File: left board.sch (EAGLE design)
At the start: 35 parts, among them IC1 LM555D, IC2 LM555D, IC3 LM50, IC4 LM50

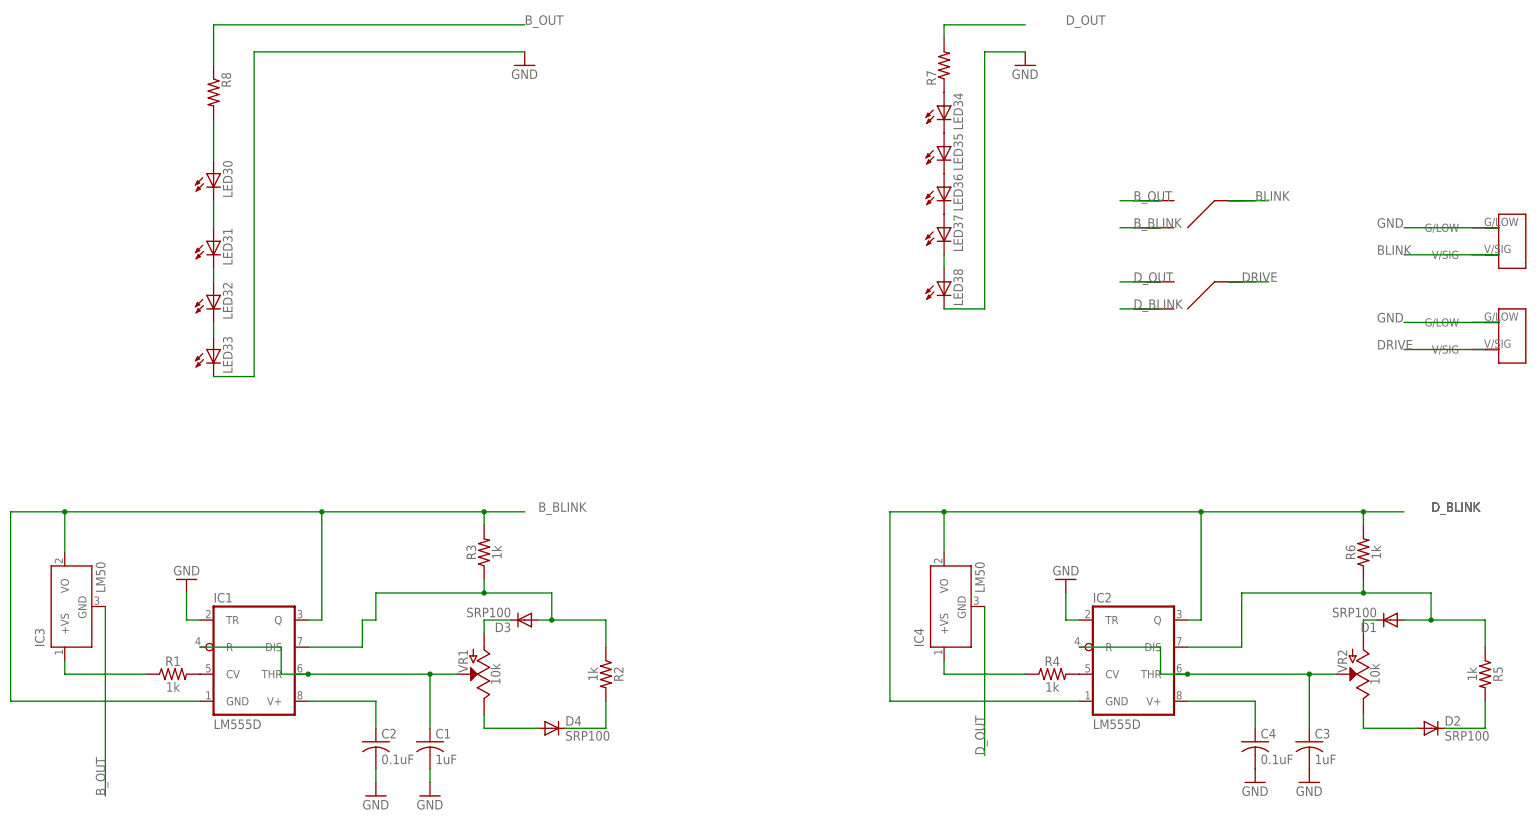
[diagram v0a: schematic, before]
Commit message: Gerbers generated
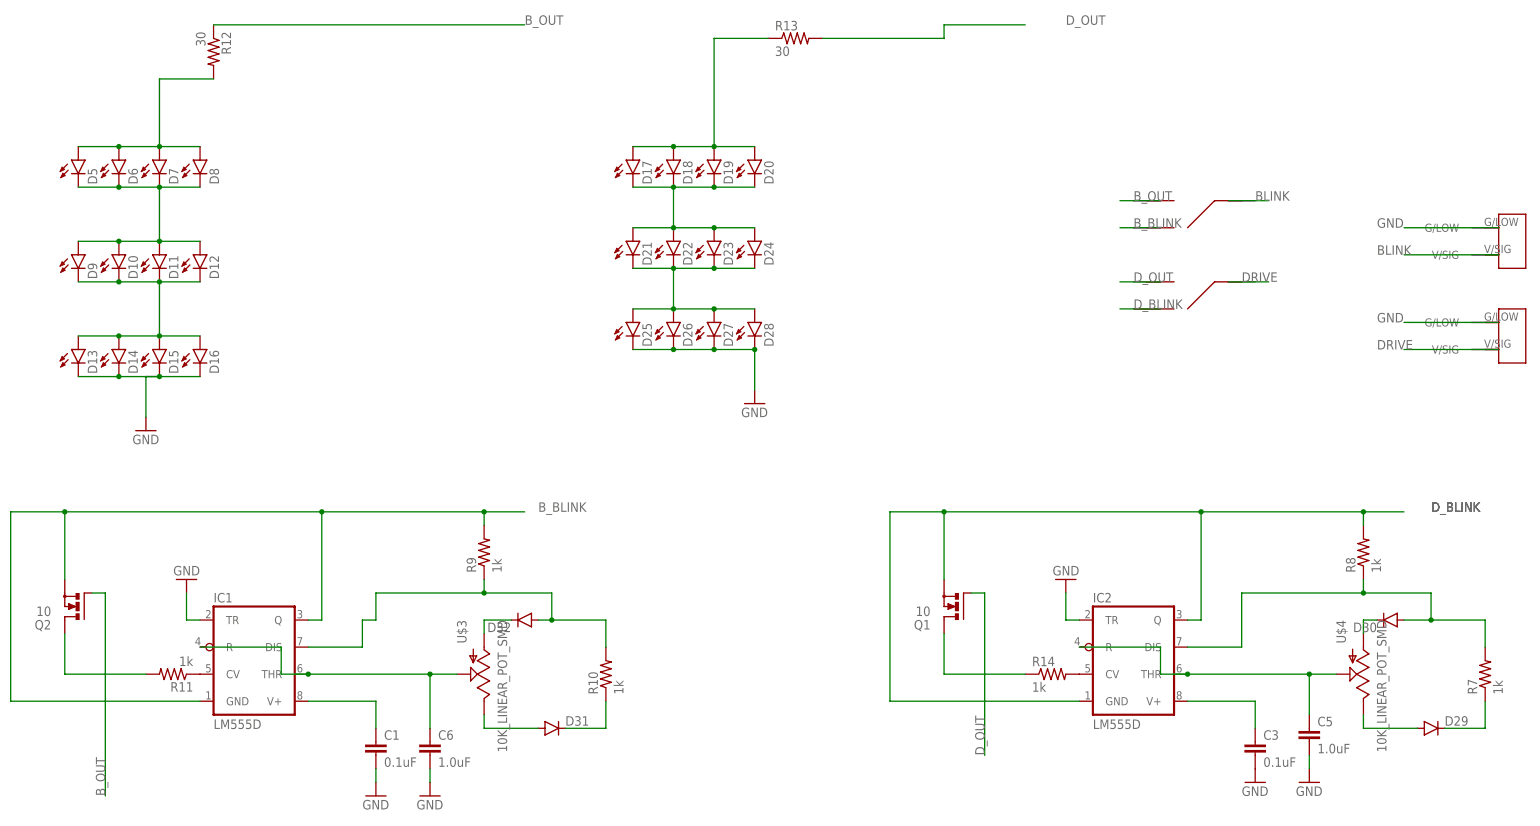
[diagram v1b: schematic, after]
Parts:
- removed C2, C4: 0.1uF, E-P-008-R1.2:C-US025-024X044
- removed D1, D2, D3, D4: SRP100, diode:SRP100
- removed IC3, IC4: LM50, linear:LM50
- removed LED30, LED31, LED32, LED33, LED34, LED35, LED36, LED37, LED38: (no value), E-P-008-R1.2:LED
- removed R1, R2, R3, R4, R5, R6: 1k, SparkFun-Resistors:1KOHM-0603-1/10W-1%
- removed VR1, VR2: 10k, SparkFun-Resistors:POTENTIOMETER-PTH-9MM-1/20W-20%
- added C5, C6: 1.0uF, SparkFun-Capacitors-extra:1.0UF-25V-+80/-20(0805)"
- added D10, D11, D12, D13, D14, D15, D16, D17, D18, D19, D20, D21, D22, D23, D24, D25, D26, D27, D28, D5, D6, D7, D8, D9: (no value), SparkFun-LED:LED5MM
- added D29, D30, D31, D32: (no value), SparkFun-DiscreteSemi:DIODESMA
- added Q1, Q2: 10, transistor-power:PMOSFET_NTO220BV
- added R10, R11, R14, R9: 1k, SparkFun-Resistors:0.22OHM-1/4W-1%(0805)
- added R12, R13: 30, SparkFun-Resistors:0.22OHM-1/4W-1%(0805)
- added U$3, U$4: 10K_LINEAR_POT_SMD, SparkFun-Resistors:10K_LINEAR_POT_SMD
- C1, C3: value 1uF -> 0.1uF; device E-P-008-R1.2:C-US025-024X044 -> SparkFun-Capacitors-extra:0.1UF-25V(+80/-20%)(0603)
- R7: value (none) -> 1k; device resistor:R-US_0204/2V -> SparkFun-Resistors:0.22OHM-1/4W-1%(0805)
- R8: value (none) -> 1k; device resistor:R-US_0204/5 -> SparkFun-Resistors:0.22OHM-1/4W-1%(0805)
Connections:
- removed net N$37: LED30.C, LED31.A
- removed net N$38: LED31.C, LED32.A
- removed net N$39: LED32.C, LED33.A
- removed net N$40: LED34.C, LED35.A
- removed net N$41: LED35.C, LED36.A
- removed net N$42: LED36.C, LED37.A
- removed net N$43: LED30.A, R8.2
- removed net N$44: LED34.A, R7.1
- removed net N$48: LED37.C, LED38.A
- new net N$12: D10.A, D11.A, D12.A, D5.C, D6.C, D7.C, D8.C, D9.A
- new net N$19: D17.A, D18.A, D19.A, D20.A, R13.1
- new net N$21: D10.C, D11.C, D12.C, D13.A, D14.A, D15.A, D16.A, D9.C
- new net N$22: D21.C, D22.C, D23.C, D24.C, D25.A, D26.A, D27.A, D28.A
- new net N$23: D17.C, D18.C, D19.C, D20.C, D21.A, D22.A, D23.A, D24.A
- new net N$8: IC2.CV, R14.2
- net B_BLINK: now also Q2.S, R9.2; no longer IC3.VO, R3.2
- net B_OUT: now also Q2.G, R12.1; no longer IC3.GND, R8.1
- net D_BLINK: now also Q1.S, R8.2; no longer IC4.VO, R6.2
- net D_OUT: now also Q1.G, R13.2; no longer IC4.GND, R7.2
- net GND: now also C5.2, C6.2, D13.C, D14.C, D15.C, D16.C, D25.C, D26.C, D27.C, D28.C; no longer C2.2, C4.2, LED33.C, LED38.C
- net N$1: now also Q2.D, R11.2; no longer IC3.+VS, R1.1
- net N$10: now also R11.1; no longer R1.2
- net N$11: now also Q1.D, R14.1; no longer IC4.+VS, R4.1
- net N$13: now also C5.1, U$4.S; no longer C3.1, VR2.S
- net N$14: now also D30.A, R7.2, R8.1; no longer D1.A, R5.1, R6.1
- net N$15: now also C3.1; no longer C4.1
- net N$16: now also D5.A, D6.A, D7.A, D8.A, R12.2; no longer IC2.CV, R4.2
- net N$17: now also D29.A, U$4.E; no longer D2.A, VR2.E
- net N$18: now also D29.C, R7.1; no longer D2.C, R5.2
- net N$2: now also D32.C, U$3.A; no longer D3.C, VR1.A
- net N$3: now also C6.1, U$3.S; no longer C1.1, VR1.S
- net N$4: now also D32.A, R10.2, R9.1; no longer D3.A, R2.1, R3.1
- net N$5: now also D31.A, U$3.E; no longer D4.A, VR1.E
- net N$6: now also C1.1; no longer C2.1
- net N$7: now also D31.C, R10.1; no longer D4.C, R2.2
- net N$9: now also D30.C, U$4.A; no longer D1.C, VR2.A
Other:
- moved on the sheet: R7, R8
